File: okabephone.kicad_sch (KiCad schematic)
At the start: 50 parts, among them J1 Micro_SD_Card_Det1, M1 Motor_DC, Q1 AO3400A, SW1 SW_MEC_5E, SW10 SW_MEC_5E, SW11 SW_MEC_5E, SW12 SW_MEC_5E, SW13 SW_MEC_5E, SW14 SW_MEC_5E, SW15 SW_MEC_5E, SW16 SW_MEC_5E, SW17 SW_MEC_5E, SW18 SW_MEC_5E, SW19 SW_MEC_5E, SW2 SW_MEC_5E, SW3 SW_MEC_5E, SW4 SW_MEC_5E, SW5 SW_MEC_5E, SW6 SW_MEC_5E, SW7 SW_MEC_5E, SW8 SW_MEC_5E, SW9 SW_MEC_5E, U1 MCP23017_ML, U2 ESP32-S3-WROOM-1, U8 PCF8563T

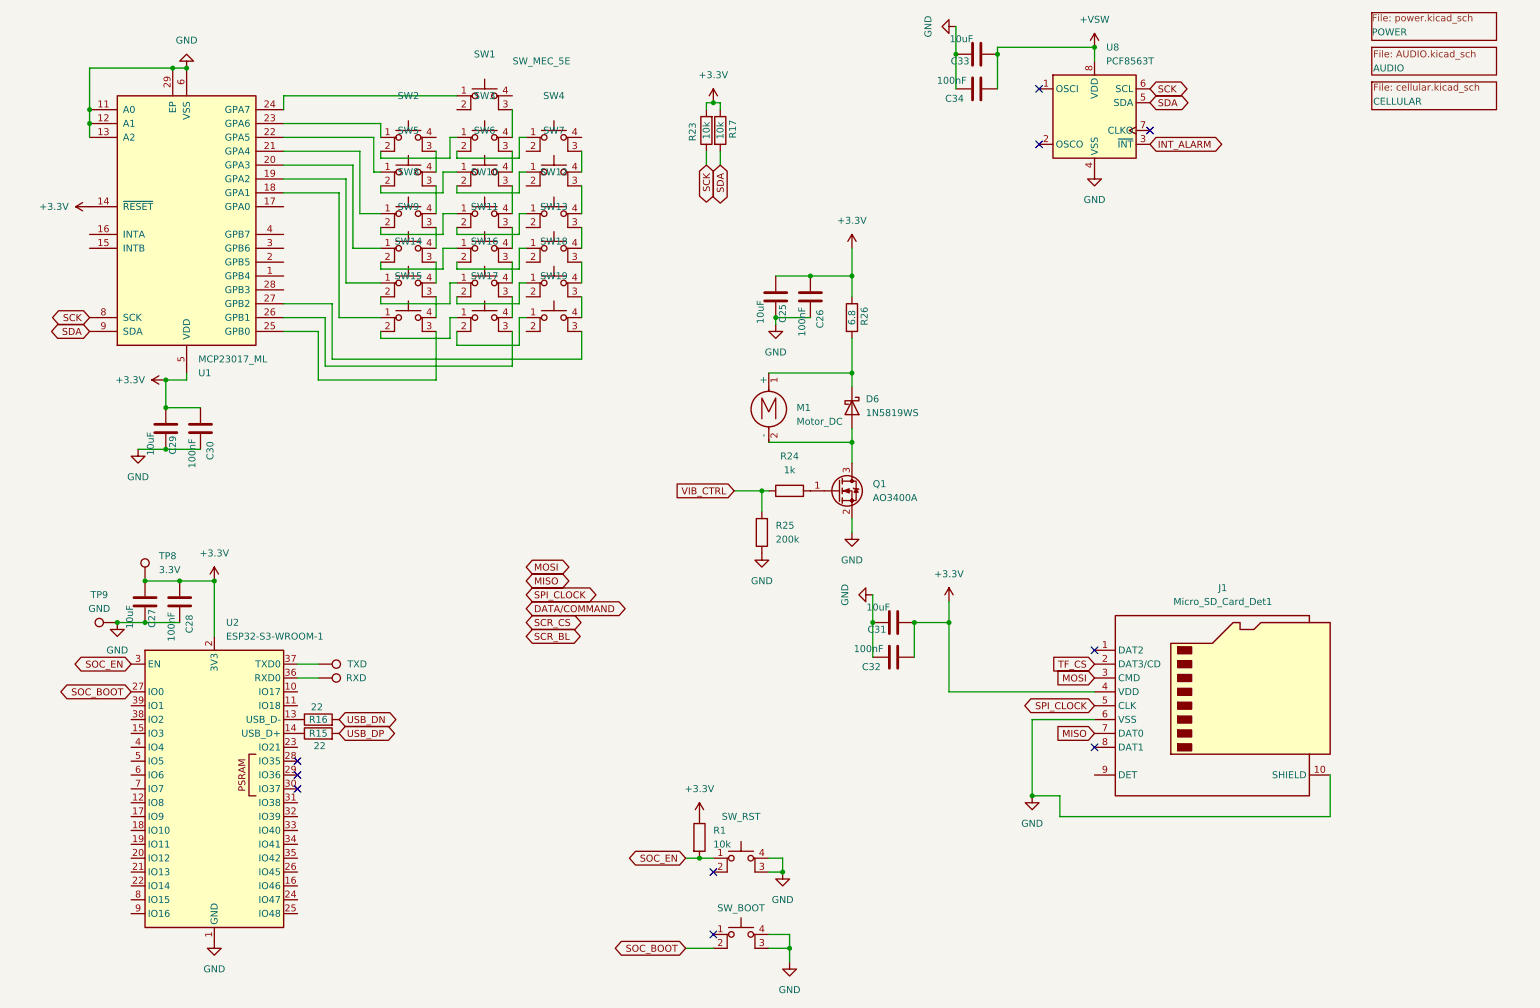
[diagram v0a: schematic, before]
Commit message: SCHEMATIC
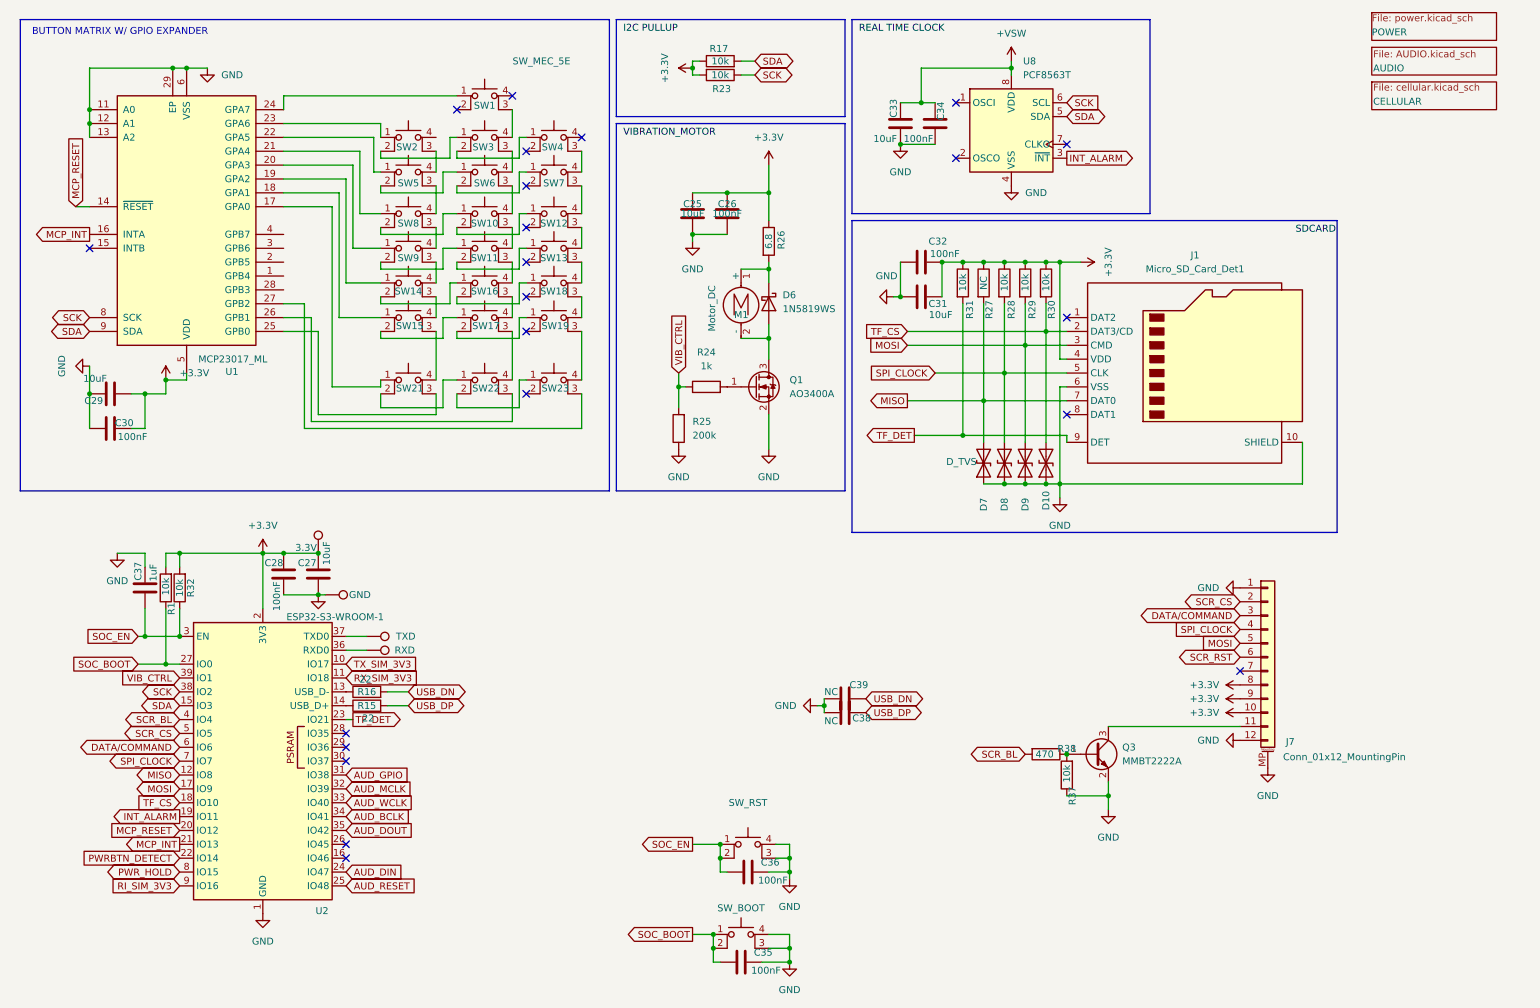
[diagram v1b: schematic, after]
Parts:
- added C35, C36: 100nF, symbol Device:C
- added C37: 1uF, symbol Device:C
- added C38, C39: NC, symbol Device:C
- added D10, D7, D8, D9: D_TVS, symbol Device:D_TVS
- added J7: Conn_01x12_MountingPin, Connector_FFC-FPC:TE_1-1734839-2_1x12-1MP_P0.5mm_Horizontal, symbol Connector_Generic_MountingPin:Conn_01x12_MountingPin
- added Q3: MMBT2222A, Package_TO_SOT_SMD:SOT-23, symbol Transistor_BJT:MMBT2222A
- added R27: NC, symbol Device:R
- added R28, R29, R30, R31, R32, R37: 10k, symbol Device:R
- added R38: 470, symbol Device:R
- added SW21, SW22, SW23: SW_MEC_5E, symbol Switch:SW_MEC_5E
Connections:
- net +3.3V: now also R1.2, J7.10 (Pin_10), J7.8 (Pin_8), J7.9 (Pin_9), R27.1, R28.1, R29.1, R30.1, R31.1, R32.2; no longer R1.1, U1.14 (~{RESET})
- net DATA/COMMAND: now also U2.6 (IO6), J7.3 (Pin_3)
- net GND: now also C35.1, C36.1, C37.1, C38.1, C39.1, D10.1 (A1), D7.1 (A1), D8.1 (A1), D9.1 (A1), J7.1 (Pin_1), J7.12 (Pin_12), J7.MP (MountPin), Q3.2 (E), R37.1
- net INT_ALARM: now also U2.19 (IO11)
- net MISO: now also U2.12 (IO8), D7.2 (A2), R27.2
- net MOSI: now also U2.17 (IO9), D9.2 (A2), J7.5 (Pin_5), R29.2
- net SCK: now also U2.38 (IO2)
- net SCR_BL: now also U2.4 (IO4), R38.2
- net SCR_CS: now also U2.5 (IO5), J7.2 (Pin_2)
- net SDA: now also U2.15 (IO3)
- net SOC_BOOT: now also R1.1, SW_BOOT.1, C35.2
- net SOC_EN: now also SW_RST.2, C36.2, C37.2, R32.1; no longer R1.2
- net SPI_CLOCK: now also U2.7 (IO7), D8.2 (A2), J7.4 (Pin_4), R28.2
- net TF_CS: now also U2.18 (IO10), D10.2 (A2), R30.2
- net USB_DN: now also C39.2
- net USB_DP: now also C38.2
- net VIB_CTRL: now also U2.39 (IO1)
- net TX_SIM_3V3: now reaches U2.10 (IO17)
- net RX_SIM_3V3: now reaches U2.11 (IO18)
- net MCP_RESET: now reaches U2.20 (IO12)
- net MCP_RESET: now also U1.14 (~{RESET})
- net MCP_INT: now reaches U2.21 (IO13)
- net MCP_INT: now also U1.16 (INTA)
- net PWRBTN_DETECT: now reaches U2.22 (IO14)
- net TF_DET: now reaches U2.23 (IO21)
- net TF_DET: now also J1.9 (DET), R31.2
- net AUD_DIN: now reaches U2.24 (IO47)
- net AUD_RESET: now reaches U2.25 (IO48)
- net AUD_GPIO: now reaches U2.31 (IO38)
- net AUD_MCLK: now reaches U2.32 (IO39)
- net AUD_WCLK: now reaches U2.33 (IO40)
- net AUD_BCLK: now reaches U2.34 (IO41)
- net AUD_DOUT: now reaches U2.35 (IO42)
- net PWR_HOLD: now reaches U2.8 (IO15)
- net RI_SIM_3V3: now reaches U2.9 (IO16)
- net at SW15.3 (K): now also SW21.4 (A); no longer U1.25 (GPB0)
- net at U1.17 (GPA0): now also SW21.1
- net at U1.26 (GPB1): now also SW22.3 (K); no longer SW17.3 (K)
- net at U1.27 (GPB2): now also SW23.3 (K); no longer SW19.3 (K)
- new net: SW21.3 (K), U1.25 (GPB0)
- new net: J7.11 (Pin_11), Q3.3 (C)
- new net: Q3.1 (B), R37.2, R38.1
- new net: SW21.2, SW22.1
- new net: SW22.2, SW23.1
- new net: SW17.3 (K), SW22.4 (A)
- new net: SW19.3 (K), SW23.4 (A)
- new net SCR_RST: J7.6 (Pin_6)
- no-connect marks 10 -> 22
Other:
- note added: "BUTTON MATRIX W/ GPIO EXPANDER"
- moved on the sheet: C25, C26, C27, C28, C29, C30, C31, C32, C33, C34, D6, J1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
